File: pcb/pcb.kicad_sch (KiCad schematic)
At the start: 66 parts, among them J1 WH, J2 RGB, J3 220, Q1 AO3400A, Q2 AO3400A, Q3 AO3400A, Q4 AO3400A, Q5 AOD452, Q6 DTD114E, Q7 AO3400A, SW1 mode, SW2 bright, T1 ., U1 ATtiny13A-SS, U2 TNY268G, U3 PC817, U4 TL431DBZ, U5 AZ1117-5.0

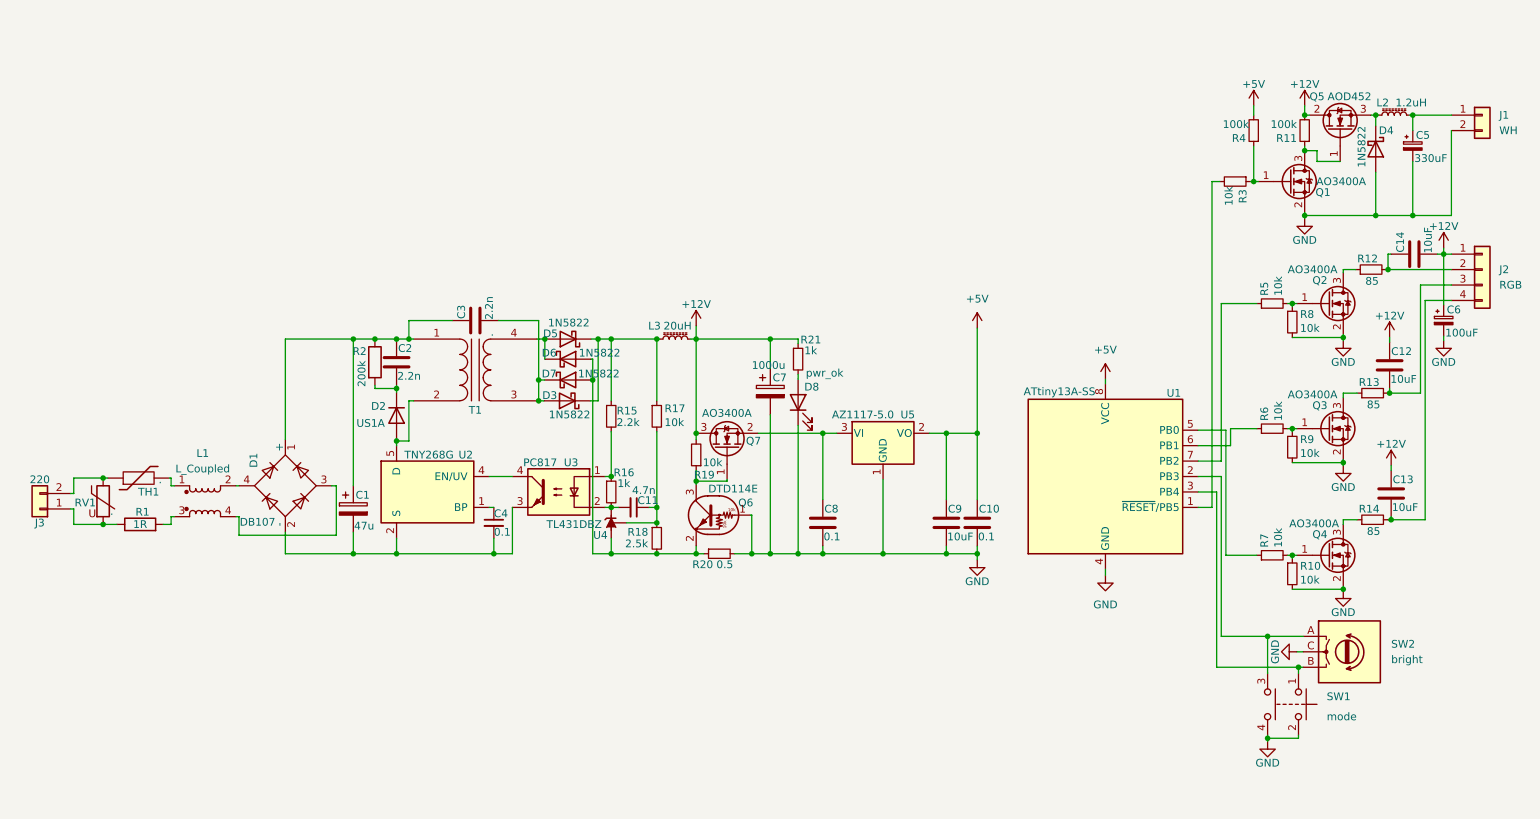
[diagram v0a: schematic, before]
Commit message: err in sch, some code added
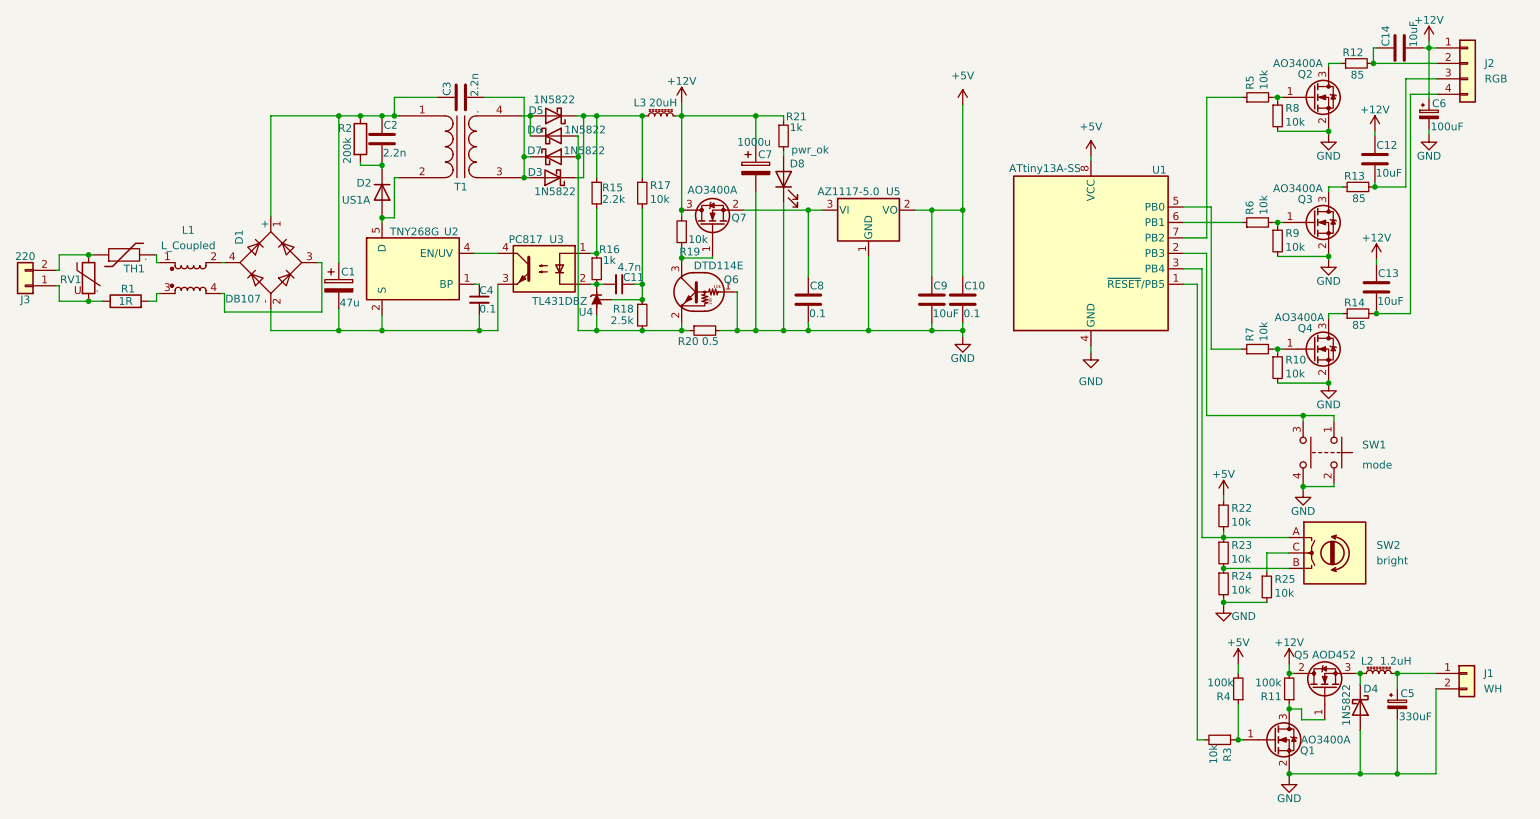
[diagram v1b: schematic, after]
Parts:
- added R22, R23, R24, R25: 10k, Resistor_SMD:R_0402_1005Metric, symbol Device:R_Small
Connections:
- net +5V: now also R22.1
- net GND: now also R24.2, R25.2; no longer SW2.C
- net at Q2.1 (G), R8.1: no longer R5.2
- net at SW1.3, U1.2 (PB3): now also SW1.1; no longer SW2.A
- new net: R22.2, R23.1, SW2.A, U1.3 (PB4)
- new net: R23.2, R24.1, SW2.B
- new net: R25.1, SW2.C
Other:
- moved on the sheet: C1, C10, C11, C12, C13, C14, C2, C3, C4, C5, C6, C7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
